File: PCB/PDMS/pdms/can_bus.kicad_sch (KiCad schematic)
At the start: 6 parts, among them U2 MCP2561-E-SN, U3 MCP2561-E-SN

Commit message: Added connector and more
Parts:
- R58, R59: footprint Resistor_SMD:R_0402_1005Metric_Pad0.72x0.64mm_HandSolder -> Resistor_SMD:R_0402_1005Metric
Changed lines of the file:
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@@
       (effects (font (size 0.8 0.8)))
     )
-    (property "Footprint" "Resistor_SMD:R_0402_1005Metric_Pad0.72x0.64mm_HandSolder" (id 2) (at 111.76 36.195 0)
+    (property "Footprint" "Resistor_SMD:R_0402_1005Metric" (id 2) (at 111.76 36.195 0)
       (effects (font (size 1.27 1.27)) hide)
     )
@@
       (effects (font (size 0.8 0.8)))
     )
-    (property "Footprint" "Resistor_SMD:R_0402_1005Metric_Pad0.72x0.64mm_HandSolder" (id 2) (at 111.76 31.75 0)
+    (property "Footprint" "Resistor_SMD:R_0402_1005Metric" (id 2) (at 111.76 31.75 0)
       (effects (font (size 1.27 1.27)) hide)
     )

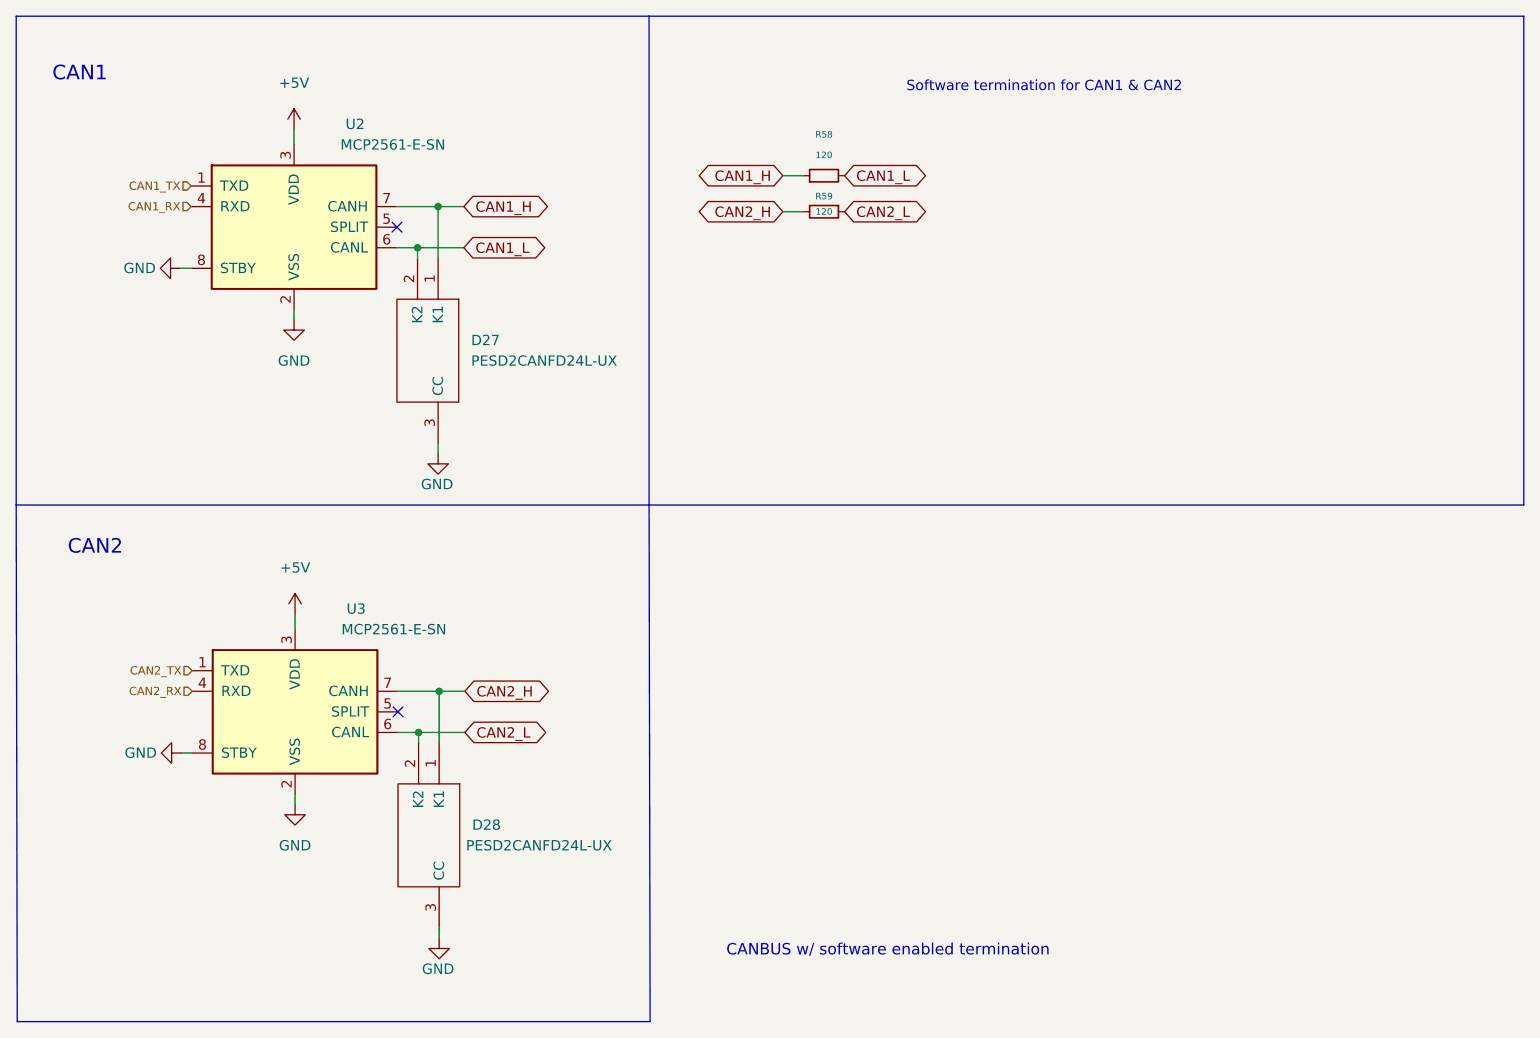
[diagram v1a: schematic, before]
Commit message: Steady layout
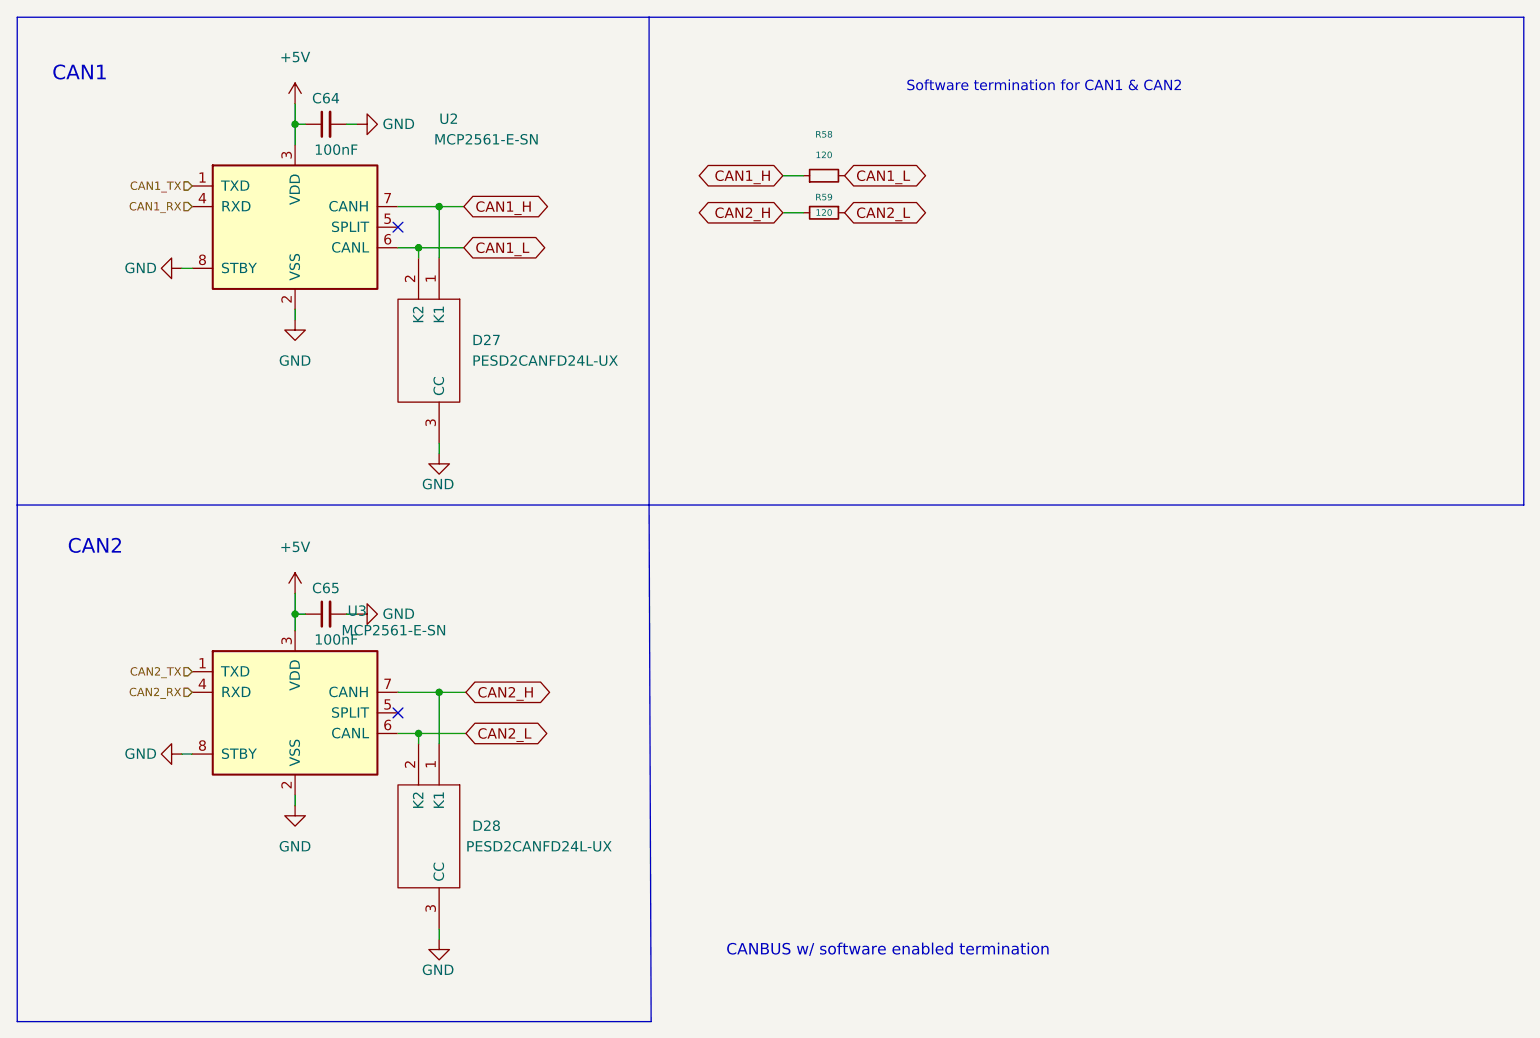
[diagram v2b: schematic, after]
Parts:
- added C64, C65: 100nF, Capacitor_SMD:C_0402_1005Metric_Pad0.74x0.62mm_HandSolder, symbol Device:C_Small
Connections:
- net +5V: now also C64.1, C65.1
- net GND: now also C64.2, C65.2
